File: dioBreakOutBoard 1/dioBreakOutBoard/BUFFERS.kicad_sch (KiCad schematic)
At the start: 24 parts, among them U5 SN74LVC8T245QPWRQ1, U6 SN74LVC8T245QPWRQ1, U7 SN74LVC8T245QPWRQ1, U8 SN74LVC8T245QPWRQ1

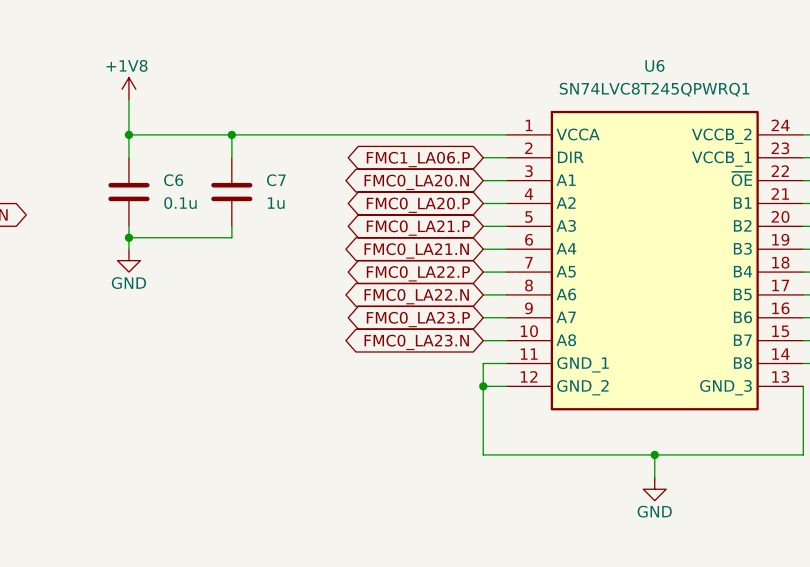
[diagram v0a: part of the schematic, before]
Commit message: More routing done
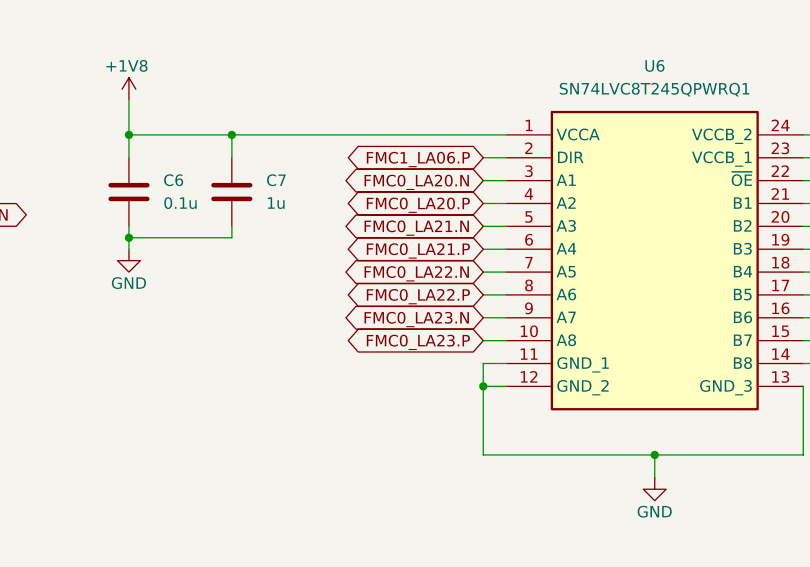
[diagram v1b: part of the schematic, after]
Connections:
- net FMC0_LA21.N: now also U6.5 (A3); no longer U6.6 (A4)
- net FMC0_LA21.P: now also U6.6 (A4); no longer U6.5 (A3)
- net FMC0_LA22.N: now also U6.7 (A5); no longer U6.8 (A6)
- net FMC0_LA22.P: now also U6.8 (A6); no longer U6.7 (A5)
- net FMC0_LA23.N: now also U6.9 (A7); no longer U6.10 (A8)
- net FMC0_LA23.P: now also U6.10 (A8); no longer U6.9 (A7)

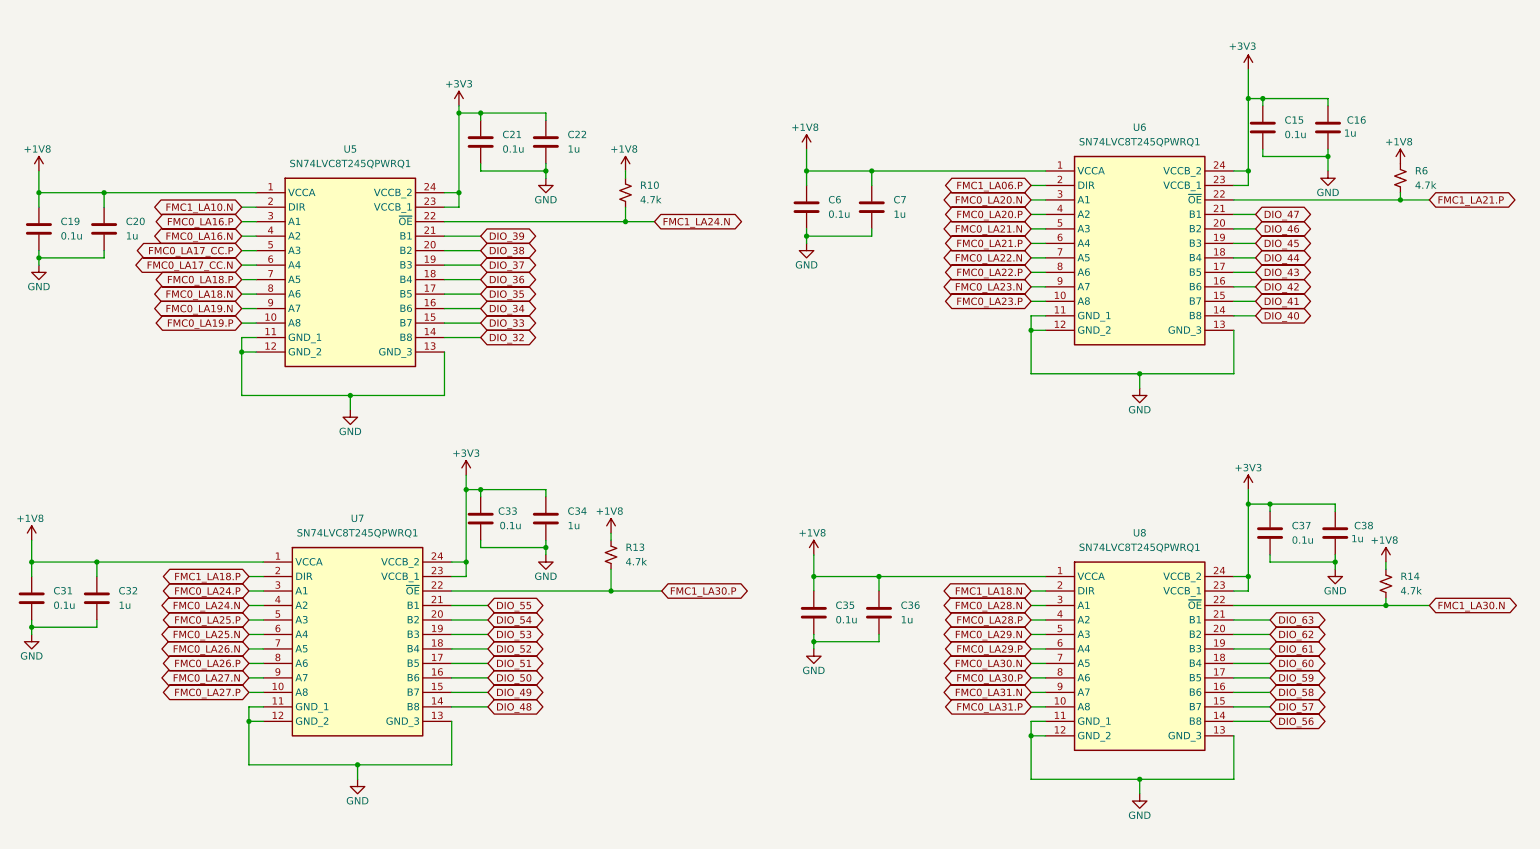
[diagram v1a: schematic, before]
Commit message: C:\Users\khernandez\KiCad\KiCad-Projects# Please enter the commit message for your changes. Lines starting
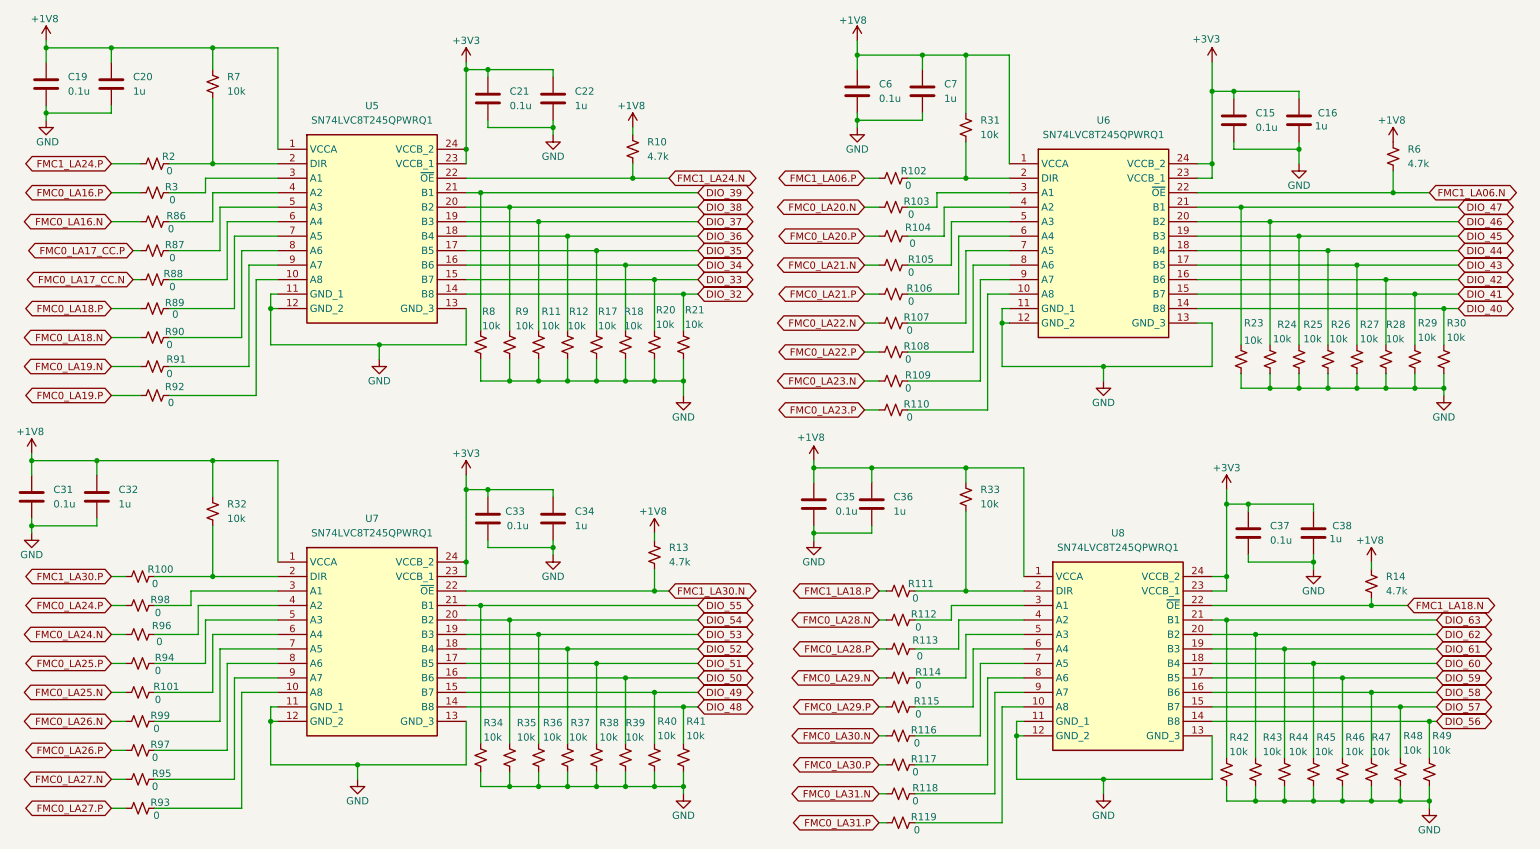
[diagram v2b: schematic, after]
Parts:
- added R100, R101, R102, R103, R104, R105, R106, R107, R108, R109, R110, R111, R112, R113, R114, R115, R116, R117, R118, R119, R2, R3, R86, R87, R88, R89, R90, R91, R92, R93, R94, R95, R96, R97, R98, R99: 0, Resistor_SMD:R_0603_1608Metric, symbol Device:R_Small_US
- added R11, R12, R17, R18, R20, R21, R23, R24, R25, R26, R27, R28, R29, R30, R31, R32, R33, R34, R35, R36, R37, R38, R39, R40, R41, R42, R43, R44, R45, R46, R47, R48, R49, R7, R8, R9: 10k, Resistor_SMD:R_0603_1608Metric, symbol Device:R_Small_US
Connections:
- net +1V8: now also R31.2, R32.2, R33.2, R7.2
- net DIO_32: now also R21.2
- net DIO_33: now also R20.2
- net DIO_34: now also R18.2
- net DIO_35: now also R17.2
- net DIO_36: now also R12.2
- net DIO_37: now also R11.2
- net DIO_38: now also R9.2
- net DIO_39: now also R8.2
- net DIO_40: now also R30.2
- net DIO_41: now also R29.2
- net DIO_42: now also R28.2
- net DIO_43: now also R27.2
- net DIO_44: now also R26.2
- net DIO_45: now also R25.2
- net DIO_46: now also R24.2
- net DIO_47: now also R23.2
- net DIO_48: now also R41.2
- net DIO_49: now also R40.2
- net DIO_50: now also R39.2
- net DIO_51: now also R38.2
- net DIO_52: now also R37.2
- net DIO_53: now also R36.2
- net DIO_54: now also R35.2
- net DIO_55: now also R34.2
- net DIO_56: now also R49.2
- net DIO_57: now also R48.2
- net DIO_58: now also R47.2
- net DIO_59: now also R46.2
- net DIO_60: now also R45.2
- net DIO_61: now also R44.2
- net DIO_62: now also R43.2
- net DIO_63: now also R42.2
- net FMC0_LA16.N: now also R86.1; no longer U5.4 (A2)
- net FMC0_LA16.P: now also R3.1; no longer U5.3 (A1)
- net FMC0_LA17_CC.N: now also R88.1; no longer U5.6 (A4)
- net FMC0_LA17_CC.P: now also R87.1; no longer U5.5 (A3)
- net FMC0_LA18.N: now also R90.1; no longer U5.8 (A6)
- net FMC0_LA18.P: now also R89.1; no longer U5.7 (A5)
- net FMC0_LA19.N: now also R91.1; no longer U5.9 (A7)
- net FMC0_LA19.P: now also R92.1; no longer U5.10 (A8)
- net FMC0_LA20.N: now also R103.1; no longer U6.3 (A1)
- net FMC0_LA20.P: now also R104.1; no longer U6.4 (A2)
- net FMC0_LA21.N: now also R105.1; no longer U6.5 (A3)
- net FMC0_LA21.P: now also R106.1; no longer U6.6 (A4)
- net FMC0_LA22.N: now also R107.1; no longer U6.7 (A5)
- net FMC0_LA22.P: now also R108.1; no longer U6.8 (A6)
- net FMC0_LA23.N: now also R109.1; no longer U6.9 (A7)
- net FMC0_LA23.P: now also R110.1; no longer U6.10 (A8)
- net FMC0_LA24.N: now also R96.1; no longer U7.4 (A2)
- net FMC0_LA24.P: now also R98.1; no longer U7.3 (A1)
- net FMC0_LA25.N: now also R101.1; no longer U7.6 (A4)
- net FMC0_LA25.P: now also R94.1; no longer U7.5 (A3)
- net FMC0_LA26.N: now also R99.1; no longer U7.7 (A5)
- net FMC0_LA26.P: now also R97.1; no longer U7.8 (A6)
- net FMC0_LA27.N: now also R95.1; no longer U7.9 (A7)
- net FMC0_LA27.P: now also R93.1; no longer U7.10 (A8)
- net FMC0_LA28.N: now also R112.1; no longer U8.3 (A1)
- net FMC0_LA28.P: now also R113.1; no longer U8.4 (A2)
- net FMC0_LA29.N: now also R114.1; no longer U8.5 (A3)
- net FMC0_LA29.P: now also R115.1; no longer U8.6 (A4)
- net FMC0_LA30.N: now also R116.1; no longer U8.7 (A5)
- net FMC0_LA30.P: now also R117.1; no longer U8.8 (A6)
- net FMC0_LA31.N: now also R118.1; no longer U8.9 (A7)
- net FMC0_LA31.P: now also R119.1; no longer U8.10 (A8)
- net FMC1_LA06.P: now also R102.1; no longer U6.2 (DIR)
- net FMC1_LA18.N: now also R14.1, U8.22 (~{OE}); no longer U8.2 (DIR)
- net FMC1_LA18.P: now also R111.1; no longer U7.2 (DIR)
- net FMC1_LA30.N: now also R13.1, U7.22 (~{OE}); no longer R14.1, U8.22 (~{OE})
- net FMC1_LA30.P: now also R100.1; no longer R13.1, U7.22 (~{OE})
- net GND: now also R11.1, R12.1, R17.1, R18.1, R20.1, R21.1, R23.1, R24.1, R25.1, R26.1, R27.1, R28.1, R29.1, R30.1, R34.1, R35.1, R36.1, R37.1, R38.1, R39.1, R40.1, R41.1, R42.1, R43.1, R44.1, R45.1, R46.1, R47.1, R48.1, R49.1, R8.1, R9.1
- net FMC1_LA10.N: no longer names the net of U5.2 (DIR)
- net FMC1_LA10.N: now also R2.2, R7.1
- net FMC1_LA21.P renamed FMC1_LA06.N
- new net: R108.2, U6.8 (A6)
- new net: R93.2, U7.10 (A8)
- new net: R110.2, U6.10 (A8)
- new net: R102.2, R31.1, U6.2 (DIR)
- new net: R109.2, U6.9 (A7)
- new net: R107.2, U6.7 (A5)
- new net: R90.2, U5.8 (A6)
- new net: R89.2, U5.7 (A5)
- new net: R98.2, U7.3 (A1)
- new net: R95.2, U7.9 (A7)
- new net: R114.2, U8.5 (A3)
- new net: R100.2, R32.1, U7.2 (DIR)
- new net: R119.2, U8.10 (A8)
- new net: R111.2, R33.1, U8.2 (DIR)
- new net: R91.2, U5.9 (A7)
- new net: R118.2, U8.9 (A7)
- new net: R103.2, U6.3 (A1)
- new net: R104.2, U6.4 (A2)
- new net: R105.2, U6.5 (A3)
- new net: R106.2, U6.6 (A4)
- new net: R92.2, U5.10 (A8)
- new net: R3.2, U5.3 (A1)
- new net: R86.2, U5.4 (A2)
- new net: R87.2, U5.5 (A3)
- new net: R88.2, U5.6 (A4)
- new net: R101.2, U7.6 (A4)
- new net: R115.2, U8.6 (A4)
- new net: R116.2, U8.7 (A5)
- new net: R96.2, U7.4 (A2)
- new net: R117.2, U8.8 (A6)
- new net: R97.2, U7.8 (A6)
- new net: R94.2, U7.5 (A3)
- new net: R99.2, U7.7 (A5)
- new net: R112.2, U8.3 (A1)
- new net: R113.2, U8.4 (A2)
- new net FMC1_LA24.P: R2.1
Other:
- moved on the sheet: C15, C16, C19, C20, C21, C22, C31, C32, C33, C34, C35, C36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

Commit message: added 2 bit buffers, which replace the previous 8 bit buffers
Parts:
- removed C6: 0.1u, Capacitor_SMD:C_0603_1608Metric, symbol Device:C
- removed R3: 0, Resistor_SMD:R_0603_1608Metric, symbol Device:R_Small_US
- removed R44: 10k, Resistor_SMD:R_0603_1608Metric, symbol Device:R_Small_US
- removed R6: 4.7k, Resistor_SMD:R_0603_1608Metric, symbol Device:R_Small_US
- removed U5, U7, U8: SN74LVC8T245QPWRQ1, SOP65P640X120-24N, symbol SN74LVC8T245QPWRQ1:SN74LVC8T245QPWRQ1
- removed U6: SN74LVC8T245QPWRQ1, LevelShifters:SOP65P640X120-24N, symbol SN74LVC8T245QPWRQ1:SN74LVC8T245QPWRQ1
- added C10, C11, C12, C23, C24, C43, C44, C45, C46, C47, C48, C55, C56, C57, C58, C63, C64, C65, C66, C8, C9: 0.1u, Capacitor_SMD:C_0603_1608Metric, symbol Device:C
- added C13, C14, C17, C18, C25, C26, C27, C28, C29, C30, C39, C40, C41, C42, C49, C50, C51, C52, C53, C54, C59, C60, C61, C62, C67, C68, C69, C70: 1u, Capacitor_SMD:C_0805_2012Metric_Pad1.18x1.45mm_HandSolder, symbol Device:C
- added IC10, IC11, IC12, IC13, IC14, IC15, IC16, IC17, IC2, IC3, IC4, IC5, IC6, IC7, IC8, IC9: SN74LVC2T45QDCURQ1, LevelShifters:SN74LVC2T45-Q1, symbol SN74LVC2T45QDCURQ1:SN74LVC2T45QDCURQ1
- added R120, R121, R122, R123, R16, R21, R22, R4, R5, R52, R53, R54, R55, R56, R57, R58, R59, R60, R61, R62, R63, R64, R66, R70, R73, R74, R75, R76, R77, R78, R79, R80, R81, R82, R83, R84, R85: 0, Resistor_SMD:R_0603_1608Metric, symbol Device:R_Small_US
- added R124, R125, R126, R127, R128, R129, R130, R131, R15, R19, R20, R51, R65, R67, R68, R69, R71, R72: 10k, Resistor_SMD:R_0603_1608Metric, symbol Device:R_Small_US
- C15, C37: value 0.1u -> 1u; footprint Capacitor_SMD:C_0603_1608Metric -> Capacitor_SMD:C_0805_2012Metric_Pad1.18x1.45mm_HandSolder; MFG_PN TMK107BJ104KA-T -> TMK212B7105KG-T
- C20, C22, C32, C34, C36, C7: value 1u -> 0.1u; footprint Capacitor_SMD:C_0805_2012Metric_Pad1.18x1.45mm_HandSolder -> Capacitor_SMD:C_0603_1608Metric; MFG_PN TMK212B7105KG-T -> TMK107BJ104KA-T
- R10, R13: value 4.7k -> 0
- R11, R12, R18, R23, R24, R26, R27, R28, R29, R30, R31, R32, R33, R34, R35, R36, R37, R38, R39, R7, R8, R9: value 10k -> 0
- R110, R111, R112, R113, R88, R89, R90, R91, R92, R93, R94, R95, R96, R97, R98, R99: value 0 -> 10k
- R14: value 4.7k -> 10k
- renumbered R20 to R44, R21 to R50, R2 to R6
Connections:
- net +1V8: now also C15.2, C16.2, C33.2, C34.2, C37.2, C38.2, R110.2, R111.2, R112.2, R113.2, R17.2, R25.2, C10.2, C11.2, C12.2, C13.2, C14.2, C17.2, C18.2, C39.2, C40.2, C41.2, C42.2, C55.2, C56.2, C57.2, C58.2, C59.2, C60.2, C61.2, C62.2, C8.2, C9.2, IC10.1 (VCCA), IC11.1 (VCCA), IC12.1 (VCCA), IC13.1 (VCCA), IC14.1 (VCCA), IC15.1 (VCCA), IC16.1 (VCCA), IC17.1 (VCCA), IC2.1 (VCCA), IC3.1 (VCCA), IC4.1 (VCCA), IC5.1 (VCCA), IC6.1 (VCCA), IC7.1 (VCCA), IC8.1 (VCCA), IC9.1 (VCCA), R15.2, R19.2, R20.2, R65.2, R67.2, R68.2, R69.2, R71.2, R72.2; no longer C19.2, C20.2, R10.2, R13.2, R31.2, R32.2, R33.2, R7.2
- net +3V3: now also C19.2, C20.2, C23.2, C24.2, C25.2, C26.2, C27.2, C28.2, C29.2, C30.2, C43.2, C44.2, C45.2, C46.2, C47.2, C48.2, C49.2, C50.2, C51.2, C52.2, C53.2, C54.2, C63.2, C64.2, C65.2, C66.2, C67.2, C68.2, C69.2, C70.2, IC10.8 (VCCB), IC11.8 (VCCB), IC12.8 (VCCB), IC13.8 (VCCB), IC14.8 (VCCB), IC15.8 (VCCB), IC16.8 (VCCB), IC17.8 (VCCB), IC2.8 (VCCB), IC3.8 (VCCB), IC4.8 (VCCB), IC5.8 (VCCB), IC6.8 (VCCB), IC7.8 (VCCB), IC8.8 (VCCB), IC9.8 (VCCB); no longer C15.2, C16.2, C33.2, C34.2, C37.2, C38.2
- net DIO_32: now also R37.2
- net DIO_33: now also R32.2
- net DIO_34: now also R34.2, R51.2; no longer R18.2
- net DIO_35: now also R30.2, R45.2; no longer R17.2
- net DIO_36: now also R38.2, R46.2; no longer R12.2
- net DIO_37: now also R31.2, R40.2; no longer R11.2
- net DIO_38: now also R35.2, R47.2; no longer R9.2
- net DIO_39: now also R29.2, R41.2; no longer R8.2
- net DIO_40: now also R39.2, R48.2; no longer R30.2
- net DIO_41: now also R33.2, R43.2; no longer R29.2
- net DIO_42: now also R49.2
- net DIO_43: now also R36.2, R42.2; no longer R27.2
- net DIO_44: now also R95.2, R82.2; no longer R26.2
- net DIO_45: now also R89.2, R76.2; no longer R25.2
- net DIO_46: now also R94.2, R83.2; no longer R24.2
- net DIO_47: now also R88.2, R77.2; no longer R23.2
- net DIO_48: now also R97.2, R85.2; no longer R41.2
- net DIO_49: now also R91.2, R79.2; no longer R40.2
- net DIO_50: now also R86.2, R98.2; no longer R39.2
- net DIO_51: now also R92.2, R80.2; no longer R38.2
- net DIO_52: now also R87.2, R99.2; no longer R37.2
- net DIO_53: now also R93.2, R81.2; no longer R36.2
- net DIO_54: now also R96.2, R84.2; no longer R35.2
- net DIO_55: now also R90.2, R78.2; no longer R34.2
- net DIO_56: now also R120.2, R128.2; no longer R49.2
- net DIO_57: now also R116.2, R124.2; no longer R48.2
- net DIO_58: now also R121.2, R129.2; no longer R47.2
- net DIO_59: now also R117.2, R125.2; no longer R46.2
- net DIO_60: now also R122.2, R130.2; no longer R45.2
- net DIO_61: now also R118.2, R126.2
- net DIO_62: now also R123.2, R131.2; no longer R43.2
- net DIO_63: now also R119.2, R127.2; no longer R42.2
- net FMC0_LA16.N: now also R24.1; no longer R86.1
- net FMC0_LA16.P: now also R13.1
- net FMC0_LA17_CC.N: now also R27.1; no longer R88.1
- net FMC0_LA17_CC.P: now also R16.1; no longer R87.1
- net FMC0_LA18.N: now also R26.1; no longer R90.1
- net FMC0_LA18.P: now also R18.1; no longer R89.1
- net FMC0_LA19.N: now also R11.1; no longer R91.1
- net FMC0_LA19.P: now also R21.1; no longer R92.1
- net FMC0_LA20.N: now also R12.1; no longer R103.1
- net FMC0_LA20.P: now also R23.1; no longer R104.1
- net FMC0_LA21.N: now also R10.1; no longer R105.1
- net FMC0_LA21.P: now also R22.1; no longer R106.1
- net FMC0_LA22.N: now also R59.1; no longer R107.1
- net FMC0_LA22.P: now also R66.1; no longer R108.1
- net FMC0_LA23.N: now also R58.1; no longer R109.1
- net FMC0_LA23.P: now also R64.1; no longer R110.1
- net FMC0_LA24.N: now also R70.1; no longer R96.1
- net FMC0_LA24.P: now also R63.1; no longer R98.1
- net FMC0_LA25.N: now also R75.1; no longer R101.1
- net FMC0_LA25.P: now also R62.1; no longer R94.1
- net FMC0_LA26.N: now also R61.1; no longer R99.1
- net FMC0_LA26.P: now also R74.1; no longer R97.1
- net FMC0_LA27.N: now also R60.1; no longer R95.1
- net FMC0_LA27.P: now also R73.1; no longer R93.1
- net FMC0_LA28.N: now also R107.1; no longer R112.1
- net FMC0_LA28.P: now also R115.1; no longer R113.1
- net FMC0_LA29.N: now also R105.1; no longer R114.1
- net FMC0_LA29.P: now also R109.1; no longer R115.1
- net FMC0_LA30.N: now also R104.1; no longer R116.1
- net FMC0_LA30.P: now also R108.1; no longer R117.1
- net FMC0_LA31.N: now also R106.1; no longer R118.1
- net FMC0_LA31.P: now also R114.1; no longer R119.1
- net FMC1_LA06.N: now also R52.2
- net FMC1_LA18.N: now also R101.1; no longer R14.1
- net FMC1_LA18.P: now also R100.1; no longer R111.1
- net FMC1_LA24.N: now also R7.1; no longer R10.1
- net FMC1_LA24.P: now also R4.1; no longer R6.1
- net FMC1_LA30.N: now also R103.1; no longer R13.1
- net FMC1_LA30.P: now also R56.1; no longer R100.1
- net GND: now also R88.1, R89.1, R90.1, R91.1, R92.1, R93.1, R94.1, R95.1, R96.1, R97.1, R98.1, R99.1, C10.1, C11.1, C12.1, C13.1, C14.1, C17.1, C18.1, C23.1, C24.1, C25.1, C26.1, C27.1, C28.1, C29.1, C30.1, C39.1, C40.1, C41.1, C42.1, C43.1, C44.1, C45.1, C46.1, C47.1, C48.1, C49.1, C50.1, C51.1, C52.1, C53.1, C54.1, C55.1, C56.1, C57.1, C58.1, C59.1, C60.1, C61.1, C62.1, C63.1, C64.1, C65.1, C66.1, C67.1, C68.1, C69.1, C70.1, C8.1, C9.1, IC10.4 (GND), IC11.4 (GND), IC12.4 (GND), IC13.4 (GND), IC14.4 (GND), IC15.4 (GND), IC16.4 (GND), IC17.4 (GND), IC2.4 (GND), IC3.4 (GND), IC4.4 (GND), IC5.4 (GND), IC6.4 (GND), IC7.4 (GND), IC8.4 (GND), IC9.4 (GND), R124.1, R125.1, R126.1, R127.1, R128.1, R129.1, R130.1, R131.1, R51.1; no longer R11.1, R12.1, R17.1, R18.1, R23.1, R24.1, R25.1, R26.1, R27.1, R28.1, R29.1, R30.1, R34.1, R35.1, R36.1, R37.1, R38.1, R39.1, R8.1, R9.1
- net at R108.2: now also IC15.3 (A2)
- net at R31.1: now also IC6.7 (B1); no longer R102.2
- net at R109.2: now also IC14.3 (A2)
- net at R107.2: now also IC17.2 (A1)
- net at R114.2: now also IC16.3 (A2)
- net at R32.1: now also IC3.7 (B1); no longer R100.2
- net at R33.1: now also IC7.7 (B1); no longer R111.2
- net at R103.2: now also R113.1, IC17.5 (DIR)
- net at R104.2: now also IC15.2 (A1)
- net at R105.2: now also IC14.2 (A1)
- net at R106.2: now also IC16.2 (A1)
- net at R6.2: now also R14.1, IC4.5 (DIR); no longer R7.1
- net at R101.2: now also R111.1, IC15.5 (DIR)
- net at R115.2: now also IC17.3 (A2)
- net FMC1_LA06.P renamed FMC1_LA26.P
- new net: IC6.5 (DIR), R15.1, R8.1
- new net: IC3.2 (A1), R11.2
- new net: IC6.6 (B2), R38.1
- new net: IC7.6 (B2), R39.1
- new net: IC12.3 (A2), R74.2
- new net: IC14.7 (B1), R118.1
- new net: IC3.5 (DIR), R20.1, R5.1
- new net: IC10.2 (A1), R63.2
- new net: IC10.3 (A2), R70.2
- new net: IC10.5 (DIR), R57.2, R65.1
- new net: IC10.6 (B2), R84.1
- new net: IC10.7 (B1), R78.1
- new net: IC4.6 (B2), R35.1
- new net: IC15.6 (B2), R121.1
- new net: IC15.7 (B1), R117.1
- new net: IC2.5 (DIR), R19.1, R4.2
- new net: IC8.5 (DIR), R52.1, R71.1
- new net: IC4.7 (B1), R29.1
- new net: IC13.5 (DIR), R56.2, R69.1
- new net: IC11.5 (DIR), R54.2, R67.1
- new net: IC13.2 (A1), R62.2
- new net: IC13.3 (A2), R75.2
- new net: IC13.6 (B2), R87.1
- new net: IC13.7 (B1), R81.1
- new net: IC12.7 (B1), R80.1
- new net: IC6.3 (A2), R27.2
- new net: IC6.2 (A1), R16.2
- new net: IC2.6 (B2), R28.1
- new net: IC7.5 (DIR), R25.1, R7.2
- new net: IC8.2 (A1), R59.2
- new net: IC5.3 (A2), R26.2
- new net: IC3.3 (A2), R21.2
- new net: IC3.6 (B2), R37.1
- new net: IC16.5 (DIR), R100.2, R110.1
- new net: IC7.2 (A1), R12.2
- new net: IC7.3 (A2), R23.2
- new net: IC17.6 (B2), R123.1
- new net: IC17.7 (B1), R119.1
- new net: IC11.2 (A1), R60.2
- new net: IC5.2 (A1), R18.2
- new net: IC9.3 (A2), R64.2
- new net: IC11.7 (B1), R79.1
- new net: IC9.7 (B1), R77.1
- new net: IC14.6 (B2), R122.1
- new net: IC8.6 (B2), R82.1
- new net: IC11.3 (A2), R73.2
- new net: IC5.5 (DIR), R17.1, R9.2
- new net: IC9.6 (B2), R83.1
- new net: IC4.2 (A1), R13.2
- new net: IC4.3 (A2), R24.2
- new net: IC8.3 (A2), R66.2
- new net: IC8.7 (B1), R76.1
- new net: IC16.7 (B1), R116.1
- new net: IC14.5 (DIR), R102.2, R112.1
- new net: IC2.2 (A1), R10.2
- new net: IC12.2 (A1), R61.2
- new net: IC12.5 (DIR), R55.2, R68.1
- new net: IC12.6 (B2), R86.1
- new net: IC9.2 (A1), R58.2
- new net: IC9.5 (DIR), R53.1, R72.1
- new net: IC2.3 (A2), R22.2
- new net: IC11.6 (B2), R85.1
- new net: IC2.7 (B1), R36.1
- new net: IC5.6 (B2), R34.1
- new net: IC16.6 (B2), R120.1
- new net: IC5.7 (B1), R30.1
- new net FMC1_LA19.N: R8.2
- new net FMC1_LA21.N: R6.1
- new net FMC1_LA21.P: R9.1
- new net FMC1_LA23.N: R55.1
- new net FMC1_LA23.P: R5.2
- new net FMC1_LA28.N: R54.1
- new net FMC1_LA28.P: R53.2
- new net FMC1_LA29.N: R57.1
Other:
- moved on the sheet: R44, R50, R6
